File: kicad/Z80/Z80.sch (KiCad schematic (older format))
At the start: 1 part

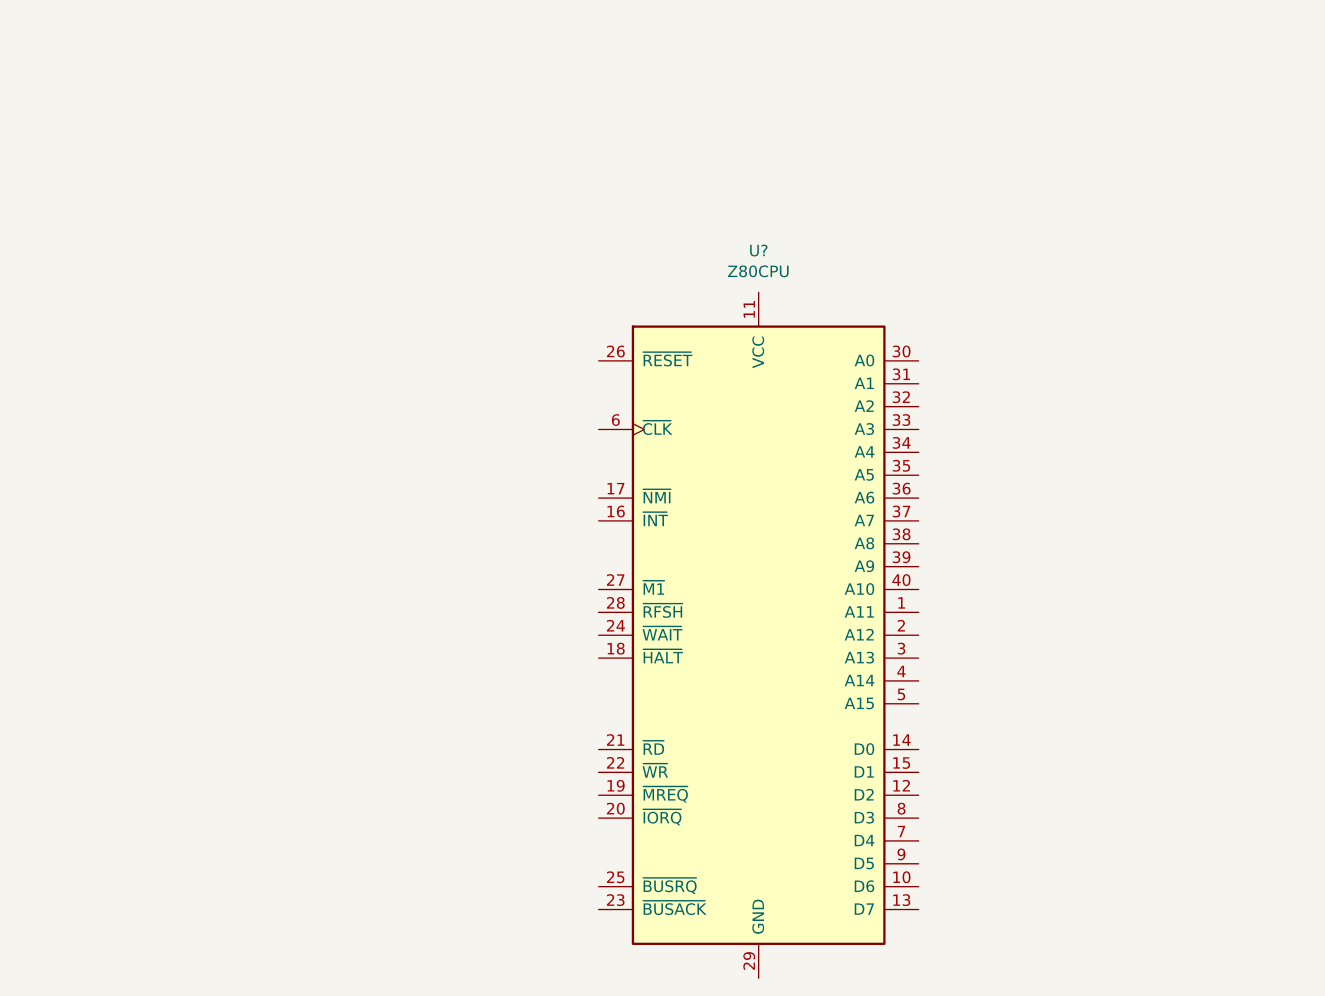
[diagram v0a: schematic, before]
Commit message: KiCAD Z80 testing
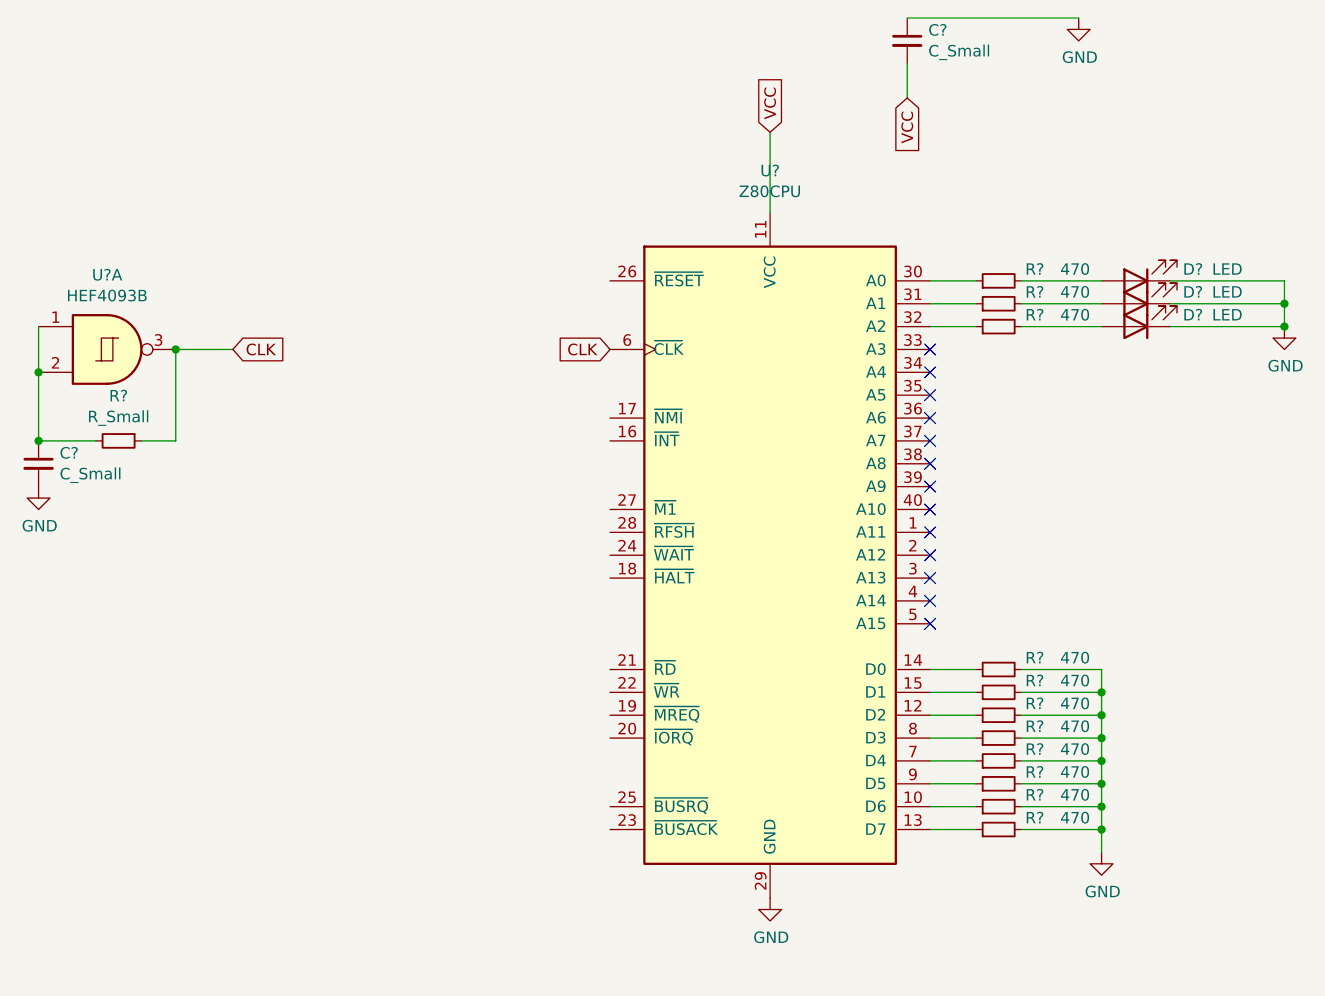
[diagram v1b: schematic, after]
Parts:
- added C? (x2): C_Small, symbol Device:C_Small
- added D? (x3): LED, symbol Device:LED
- added R?: R_Small, symbol Device:R_Small
- added R? (x11): 470, symbol Device:R_Small
- added U?: HEF4093B, symbol 4xxx:HEF4093B
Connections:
- net at U?.10 (D6): now also R?.1
- net VCC: now reaches U?.11 (VCC)
- net VCC: now also C?.2
- net at U?.12 (D2): now also R?.1
- net at U?.13 (D7): now also R?.1
- net at U?.14 (D0): now also R?.1
- net at U?.15 (D1): now also R?.1
- net GND: now reaches U?.29 (GND)
- net GND: now also C?.1, C?.2, D?.1 (K), D?.1 (K), D?.1 (K), R?.2, R?.2, R?.2, R?.2, R?.2, R?.2, R?.2, R?.2
- net at U?.30 (A0): now also R?.1
- net at U?.31 (A1): now also R?.1
- net at U?.32 (A2): now also R?.1
- net CLK: now reaches U?.6 (~CLK~)
- net CLK: now also R?.1, U?.3
- net at U?.7 (D4): now also R?.1
- net at U?.8 (D3): now also R?.1
- net at U?.9 (D5): now also R?.1
- new net: C?.1, R?.2, U?.1, U?.2
- new net: D?.2 (A), R?.2 (x3)
- no-connect marks 0 -> 13
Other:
- moved on the sheet: U?
